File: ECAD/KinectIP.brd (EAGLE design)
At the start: 64.8 x 59.4 mm, 13 parts, among them P5+ 2PIN-FEMALE-HEADER

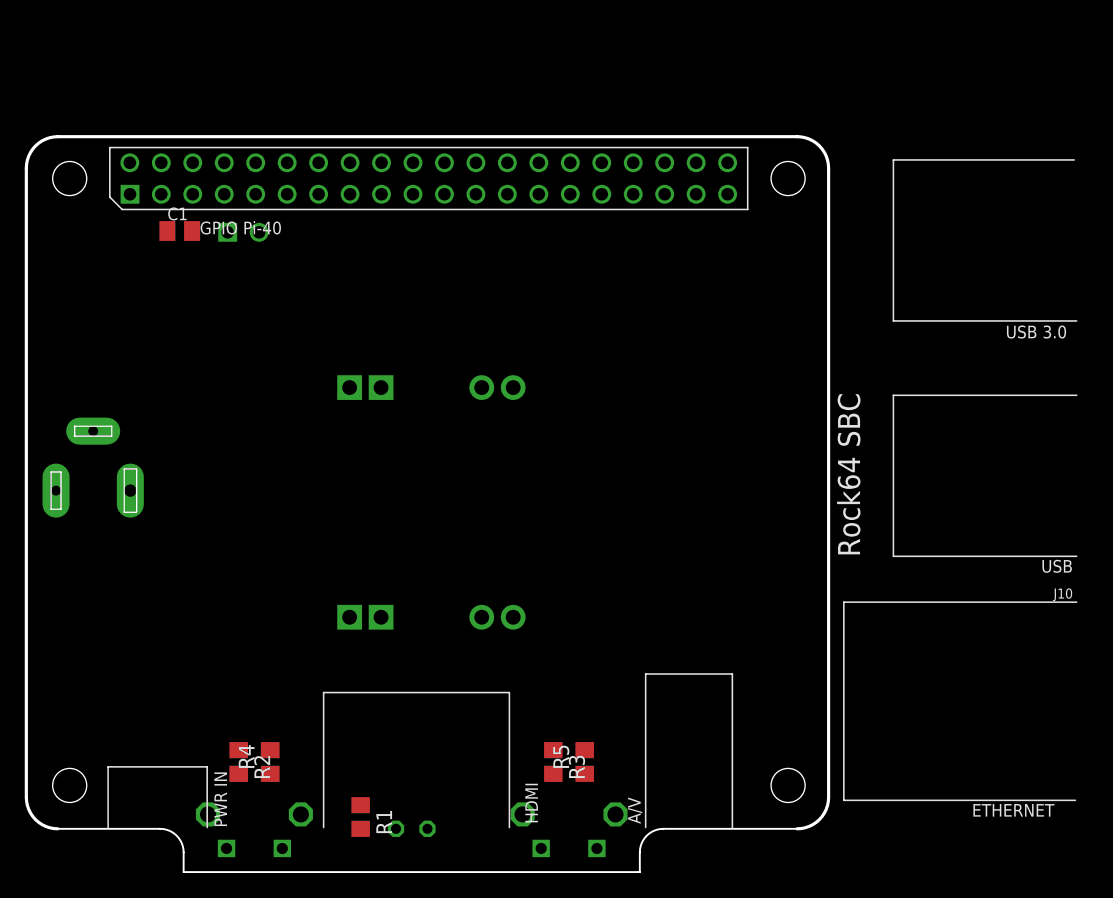
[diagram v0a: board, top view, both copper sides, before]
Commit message: update ECAD
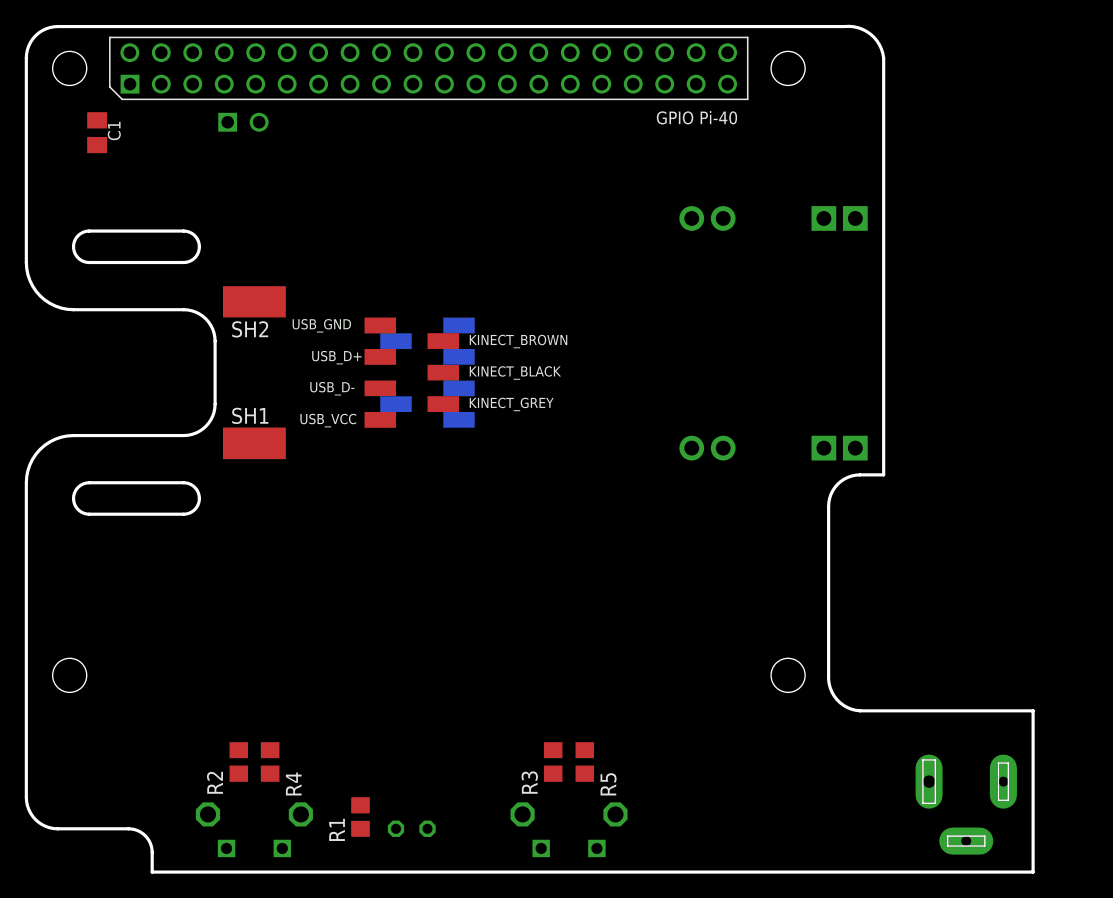
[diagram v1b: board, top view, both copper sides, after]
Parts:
- added KINECT_BLACK, KINECT_BROWN, KINECT_GREY, USB3_BLUE, USB3_GND1, USB3_GND2, USB3_ORANGE, USB3_PURPLE, USB3_YELLOW, USB_D+, USB_D-, USB_GND, USB_VCC: (no value), wirepad:SMD1,27-2,54
- added SH1, SH2: GND, wirepad:SMD2,54-5,08
- moved J1 74.3 mm to (75.9, 8.89), turned to 0 degrees
- moved 12V->5V 30.8 mm to (60.3, 45.1), turned to 270 degrees
- moved C1 10.4 mm to (5.71, 61.3), turned to 270 degrees
- moved P5+ 8.89 mm to (16.3, 62.1)
- moved PCB2 8.89 mm to (0.00, 14.0)
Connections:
- net +12V: now also KINECT_BROWN.1
- net 0V: now also KINECT_BLACK.1, KINECT_GREY.1, SH1.1, SH2.1
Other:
- board size 64.8 x 59.4 mm -> 81.3 x 68.3 mm
